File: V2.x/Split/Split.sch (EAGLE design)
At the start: 6 parts, among them J1 3-794618-4, J2 3-794618-4, J3 3-794618-4, X2 2X1-A

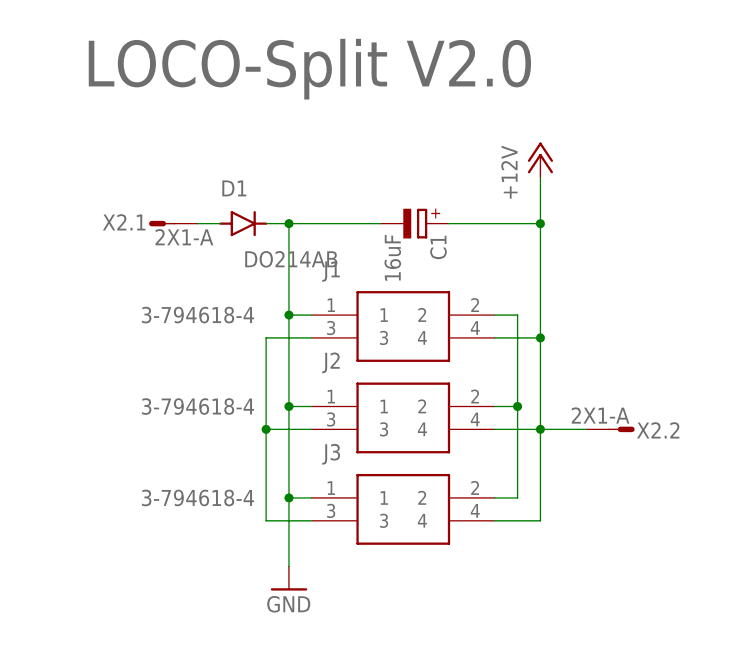
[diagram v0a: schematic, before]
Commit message: initial
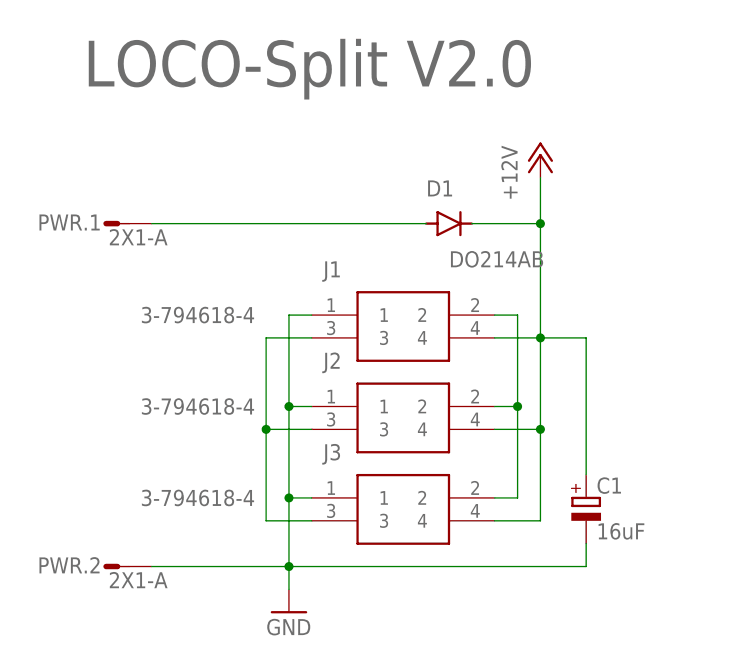
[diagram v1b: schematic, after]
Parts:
- removed X2: 2X1-A, con-amp-micro-mate-n-lock:2X1-A
- added PWR: 2X1-A, con-amp-micro-mate-n-lock:2X1-A
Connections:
- net +12V: now also D1.C; no longer X2.2.S
- net GND: now also PWR.2.S; no longer D1.C
- net N$1: now also PWR.1.S; no longer X2.1.S
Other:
- moved on the sheet: C1, D1
